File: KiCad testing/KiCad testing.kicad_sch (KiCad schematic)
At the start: 40 parts, among them J1 USB_A, Q1 IRF540N, Q2 IRF540N, Q3 IRF540N, Q4 IRF540N, U1 IR2213, U4 IR2213

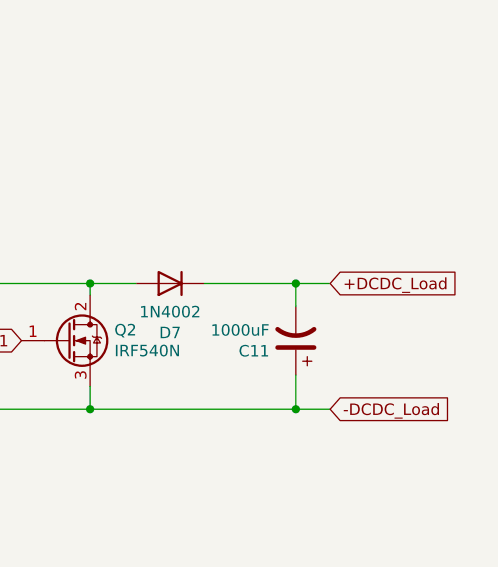
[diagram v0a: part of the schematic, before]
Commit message: update pcb
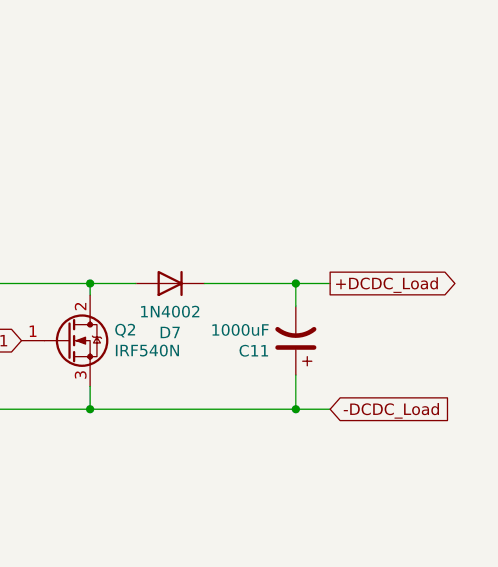
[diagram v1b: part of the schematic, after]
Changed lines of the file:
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@@
     )
   )
-  (global_label "+DCDC_Load" (shape input) (at 251.46 81.28 0) (fields_autoplaced)
+  (global_label "+DCDC_Load" (shape output) (at 251.46 81.28 0) (fields_autoplaced)
     (effects (font (size 1.27 1.27)) (justify left))
     (property "Intersheetrefs" "${INTERSHEET_REFS}" (at 265.8861 81.28 0)
